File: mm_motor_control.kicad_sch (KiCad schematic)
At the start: 0 parts

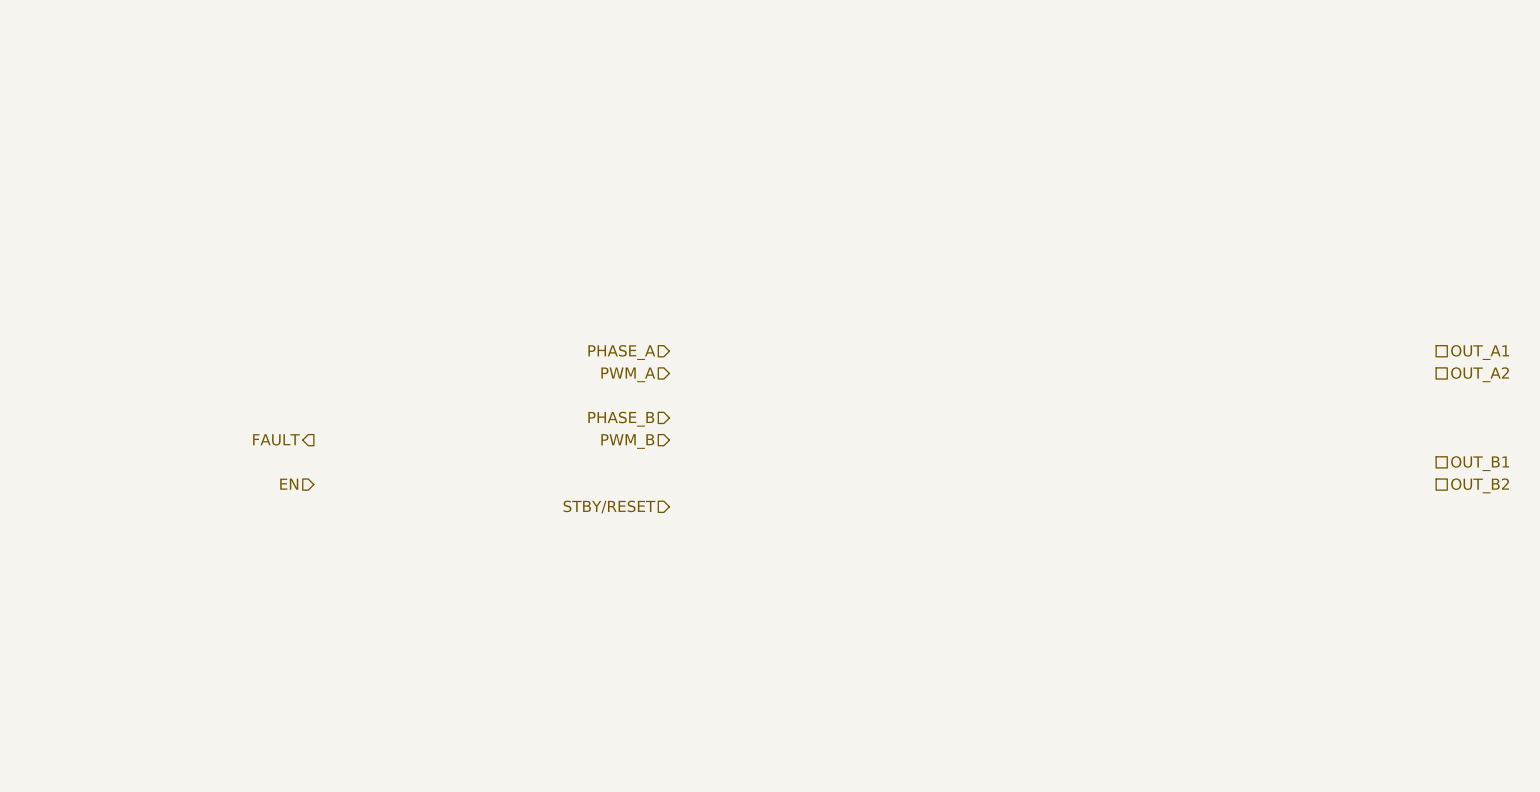
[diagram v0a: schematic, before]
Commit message: fin tp2
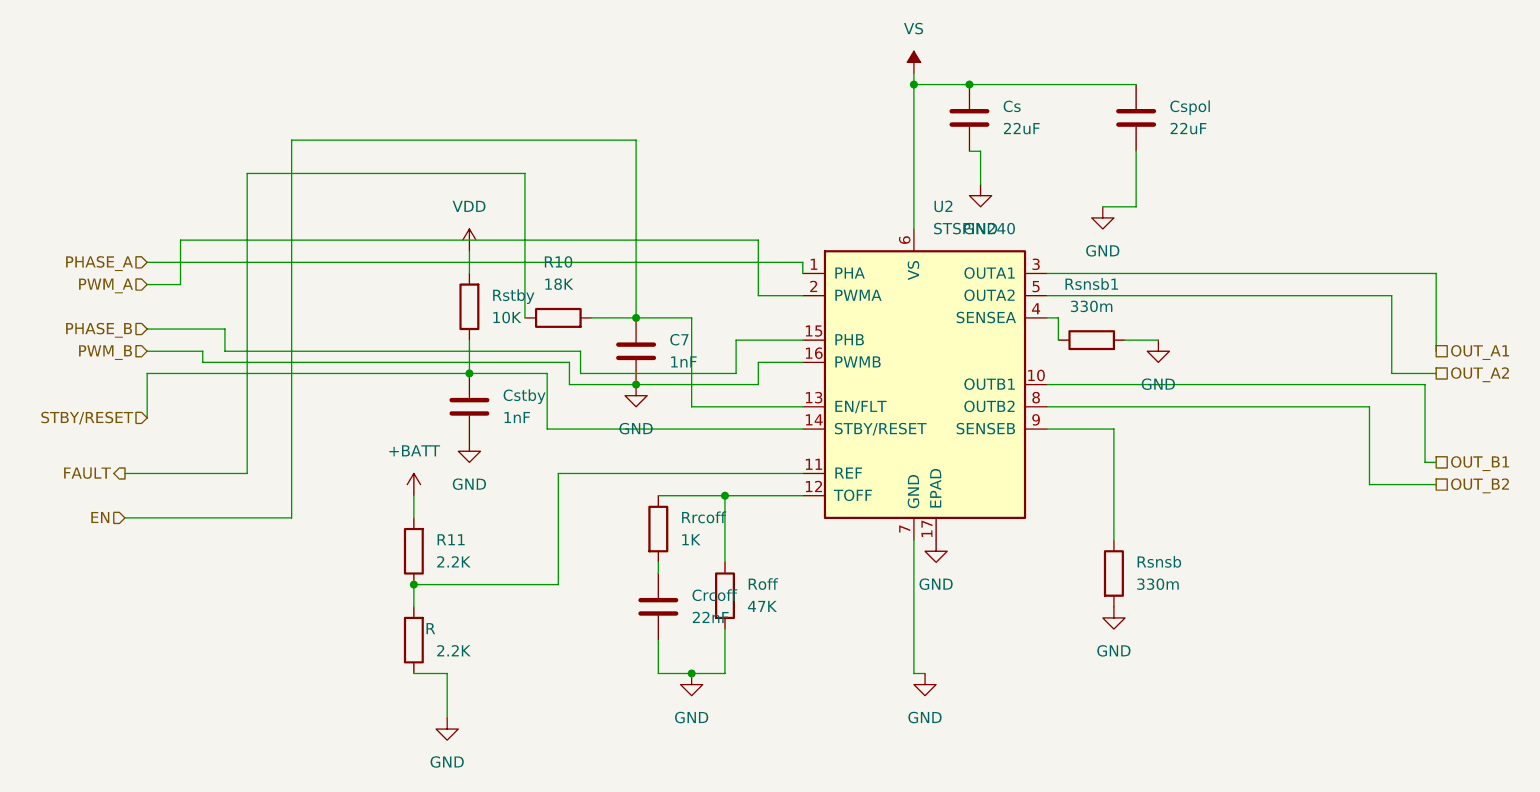
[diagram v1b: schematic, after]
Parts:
- added C7, Cstby: 1nF, symbol Device:C
- added Crcoff: 22nF, symbol Device:C
- added Cs, Cspol: 22uF, symbol Device:C
- added R, R11: 2.2K, symbol Device:R
- added R10: 18K, symbol Device:R
- added Roff: 47K, symbol Device:R
- added Rrcoff: 1K, symbol Device:R
- added Rsnsb, Rsnsb1: 330m, symbol Device:R
- added Rstby: 10K, symbol Device:R
- added U2: STSPIN240, Package_DFN_QFN:VQFN-16-1EP_3x3mm_P0.5mm_EP1.8x1.8mm, symbol Driver_Motor:STSPIN240
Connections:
- net EN: now also C7.2, R10.2, U2.13 (EN/FLT)
- net FAULT: now also R10.1
- net OUT_A1: now also U2.3 (OUTA1)
- net OUT_A2: now also U2.5 (OUTA2)
- net OUT_B1: now also U2.10 (OUTB1)
- net OUT_B2: now also U2.8 (OUTB2)
- net PHASE_A: now also U2.1 (PHA)
- net PHASE_B: now also U2.15 (PHB)
- net PWM_A: now also U2.2 (PWMA)
- net STBY/RESET: now also Cstby.2, Rstby.1, U2.14 (STBY/RESET)
- new net: R.2, R11.1, U2.11 (REF)
- new net: Roff.1, Rrcoff.1, U2.12 (TOFF)
- new net: Crcoff.2, Rrcoff.2
- new net: Rsnsb1.1, U2.4 (SENSEA)
- new net: Rsnsb.1, U2.9 (SENSEB)
- new net +BATT: R11.2
- new net GND: C7.1, Crcoff.1, Cs.2, Cspol.1, Cstby.1, R.1, Roff.2, Rsnsb.2, Rsnsb1.2, U2.16 (PWMB), U2.17 (EPAD), U2.7 (GND)
- new net VDD: Rstby.2
- new net VS: Cs.1, Cspol.2, U2.6 (VS)
